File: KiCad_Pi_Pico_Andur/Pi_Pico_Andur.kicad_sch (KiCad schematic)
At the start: 1 part

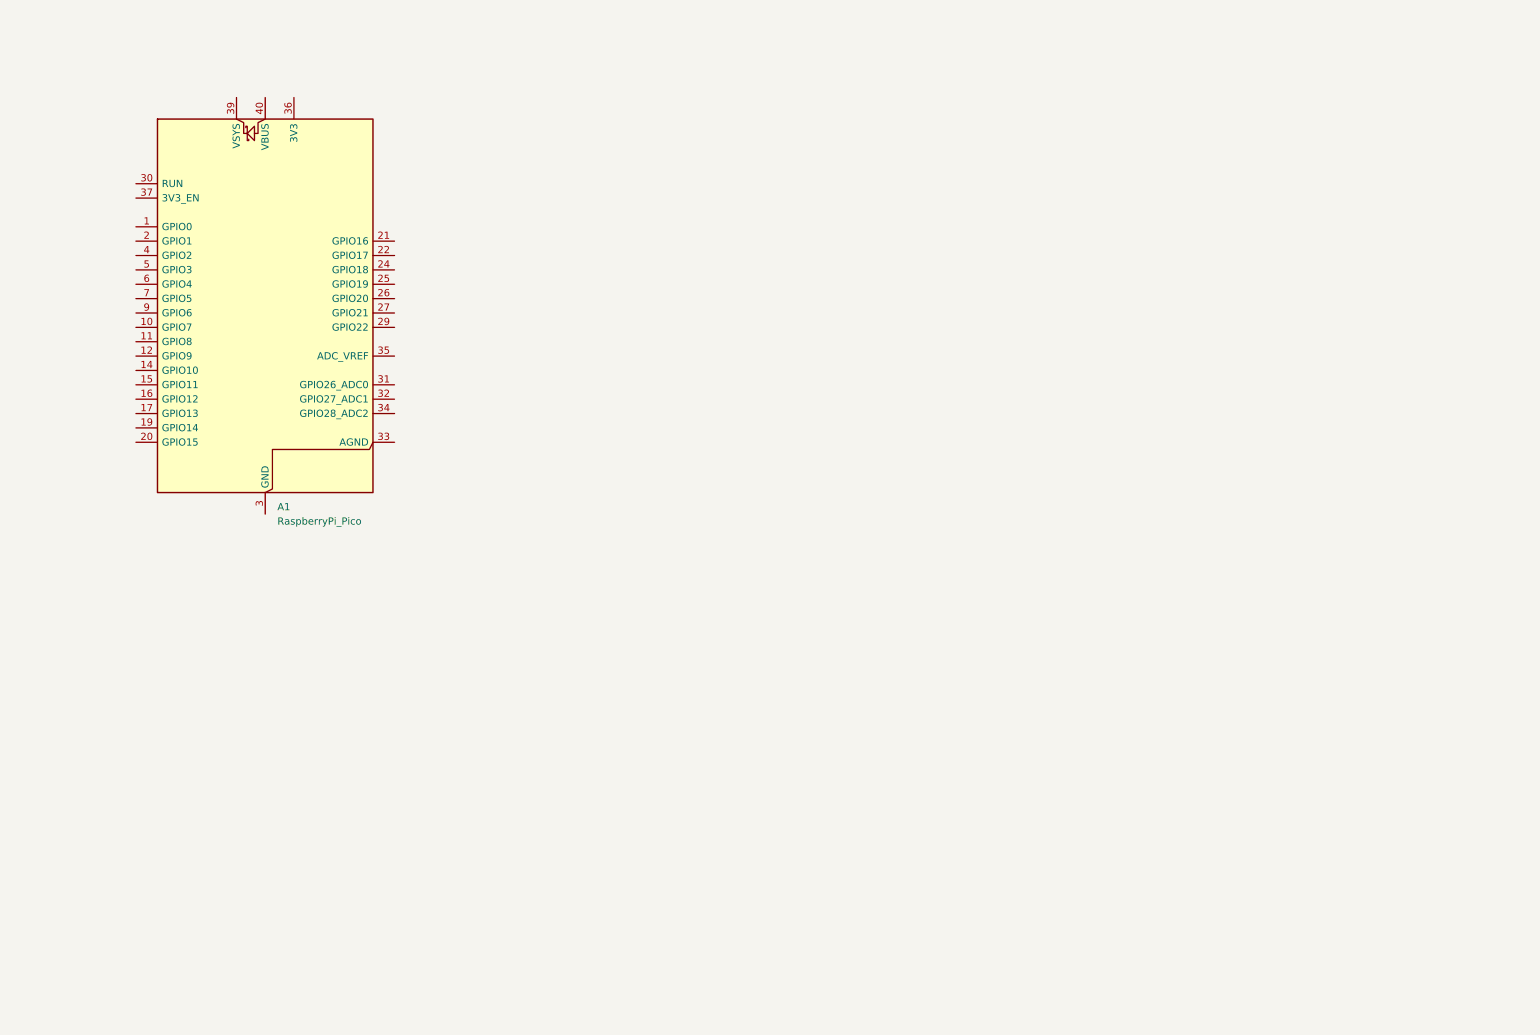
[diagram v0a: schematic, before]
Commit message: kicad
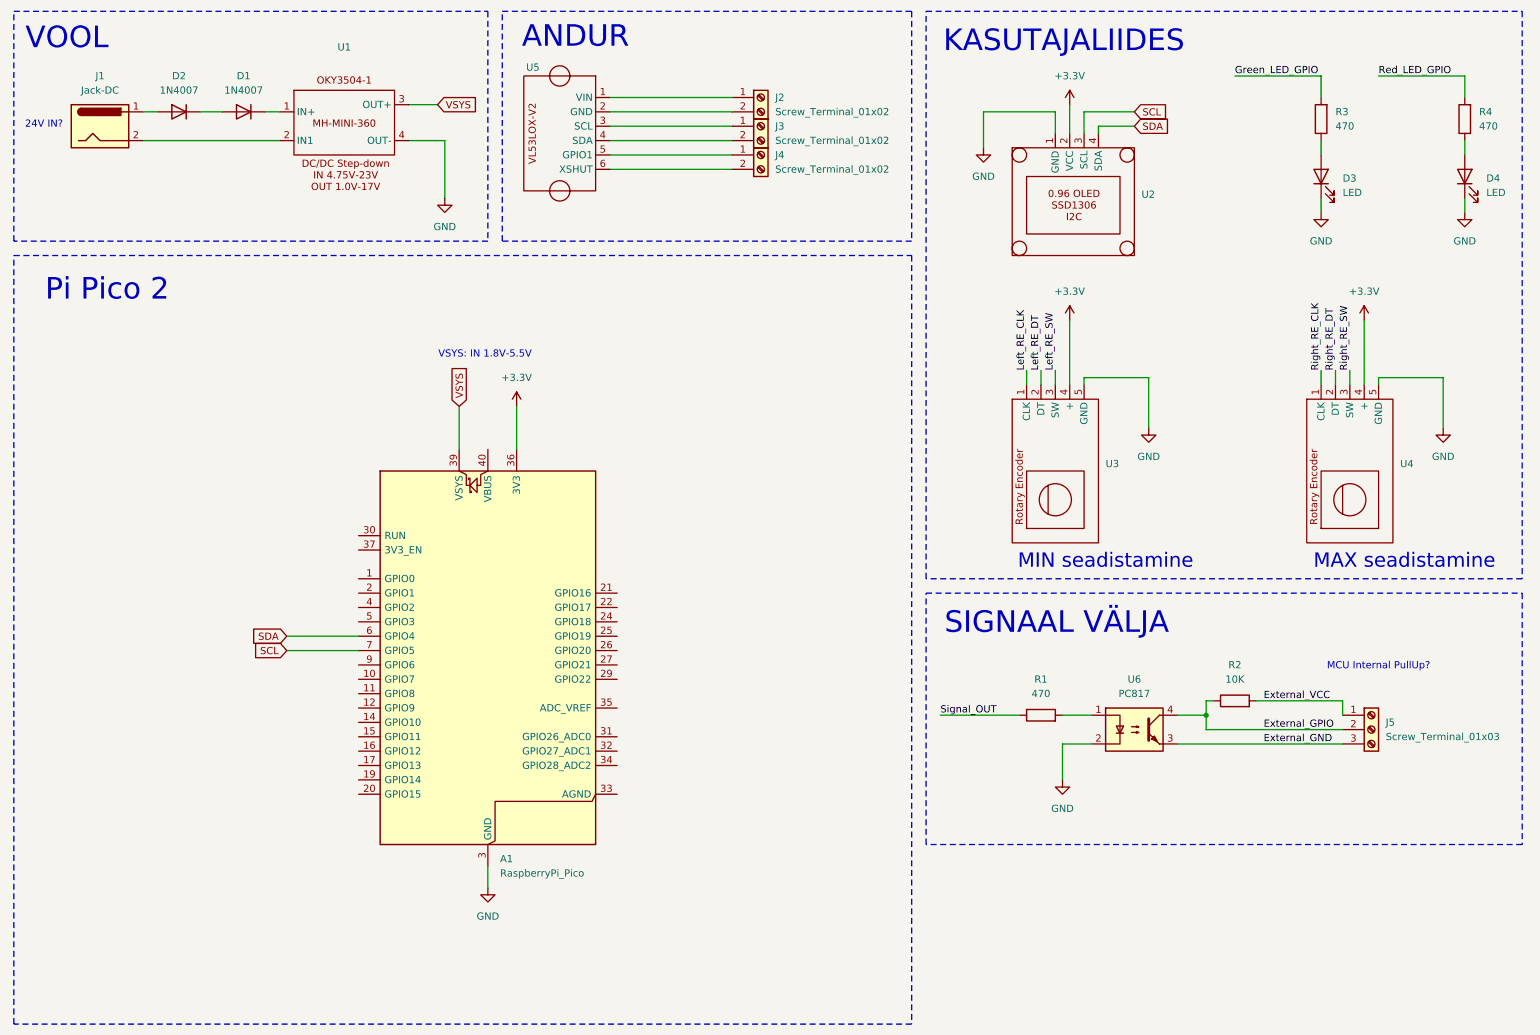
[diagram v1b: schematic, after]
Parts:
- added D1, D2: 1N4007, Diode_THT:D_DO-41_SOD81_P10.16mm_Horizontal, symbol Diode:1N4007
- added D3, D4: LED, symbol Device:LED
- added J1: Jack-DC, symbol Connector:Jack-DC
- added J2, J3, J4: Screw_Terminal_01x02, TerminalBlock:TerminalBlock_MaiXu_MX126-5.0-02P_1x02_P5.00mm, symbol Connector:Screw_Terminal_01x02
- added J5: Screw_Terminal_01x03, symbol Connector:Screw_Terminal_01x03
- added R1, R3, R4: 470, symbol Device:R
- added R2: 10K, symbol Device:R
- added U1: ~, symbol Tauno_Library:Tauno_OKY3504-1
- added U2: ~, symbol Tauno_Library:Tauno_Oled_096_SSD1306
- added U3, U4: ~, symbol Tauno_Library:Tauno_Rotary_Encoder
- added U5: ~, symbol Tauno_Library:Tauno_TOF_VL53LOX
- added U6: PC817, Package_DIP:DIP-4_W7.62mm, symbol Isolator:PC817
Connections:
- net GND: now reaches A1.13 (GND), A1.18 (GND), A1.23 (GND), A1.28 (GND), A1.3 (GND), A1.38 (GND), A1.8 (GND)
- net GND: now also D3.1 (K), D4.1 (K), U1.4 (OUT-), U2.1 (GND), U3.5 (GND), U4.5 (GND), U6.2
- net +3.3V: now reaches A1.36 (3V3)
- net +3.3V: now also U2.2 (VCC), U3.4 (+), U4.4 (+)
- net VSYS: now reaches A1.39 (VSYS)
- net VSYS: now also U1.3 (OUT+)
- net SDA: now reaches A1.6 (GPIO4)
- net SDA: now also U2.4 (SDA)
- net SCL: now reaches A1.7 (GPIO5)
- net SCL: now also U2.3 (SCL)
- new net: R1.2, U6.1
- new net: D4.2 (A), R4.1
- new net: D1.2 (A), D2.1 (K)
- new net: D2.2 (A), J1.1
- new net: D1.1 (K), U1.1 (IN+)
- new net: J1.2, U1.2 (IN1)
- new net: J2.1 (Pin_1), U5.1 (VIN)
- new net: J2.2 (Pin_2), U5.2 (GND)
- new net: D3.2 (A), R3.1
- new net: J4.1 (Pin_1), U5.5 (GPIO1)
- new net: J4.2 (Pin_2), U5.6 (XSHUT)
- new net: J3.1 (Pin_1), U5.3 (SCL)
- new net: J3.2 (Pin_2), U5.4 (SDA)
- new net External_GND: J5.3 (Pin_3), U6.3
- new net External_GPIO: J5.2 (Pin_2), R2.1, U6.4
- new net External_VCC: J5.1 (Pin_1), R2.2
- new net Green_LED_GPIO: R3.2
- new net Left_RE_CLK: U3.1 (CLK)
- new net Left_RE_DT: U3.2 (DT)
- new net Left_RE_SW: U3.3 (SW)
- new net Red_LED_GPIO: R4.2
- new net Right_RE_CLK: U4.1 (CLK)
- new net Right_RE_DT: U4.2 (DT)
- new net Right_RE_SW: U4.3 (SW)
- new net Signal_OUT: R1.1
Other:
- note added: "24V IN?"
- note added: "ANDUR"
- note added: "KASUTAJALIIDES"
- note added: "MAX seadistamine"
- note added: "MCU Internal PullUp?"
- note added: "MIN seadistamine"
- note added: "Pi Pico 2"
- note added: "SIGNAAL VÄLJA"
- note added: "VOOL"
- note added: "VSYS: IN 1.8V-5.5V"
- moved on the sheet: A1
